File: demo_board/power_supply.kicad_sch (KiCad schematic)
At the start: 23 parts, among them J2 USB_C_Receptacle_USB2.0_16P, J3 BATT, U2 MCP73871-2CC, U3 AP2112K-3.3

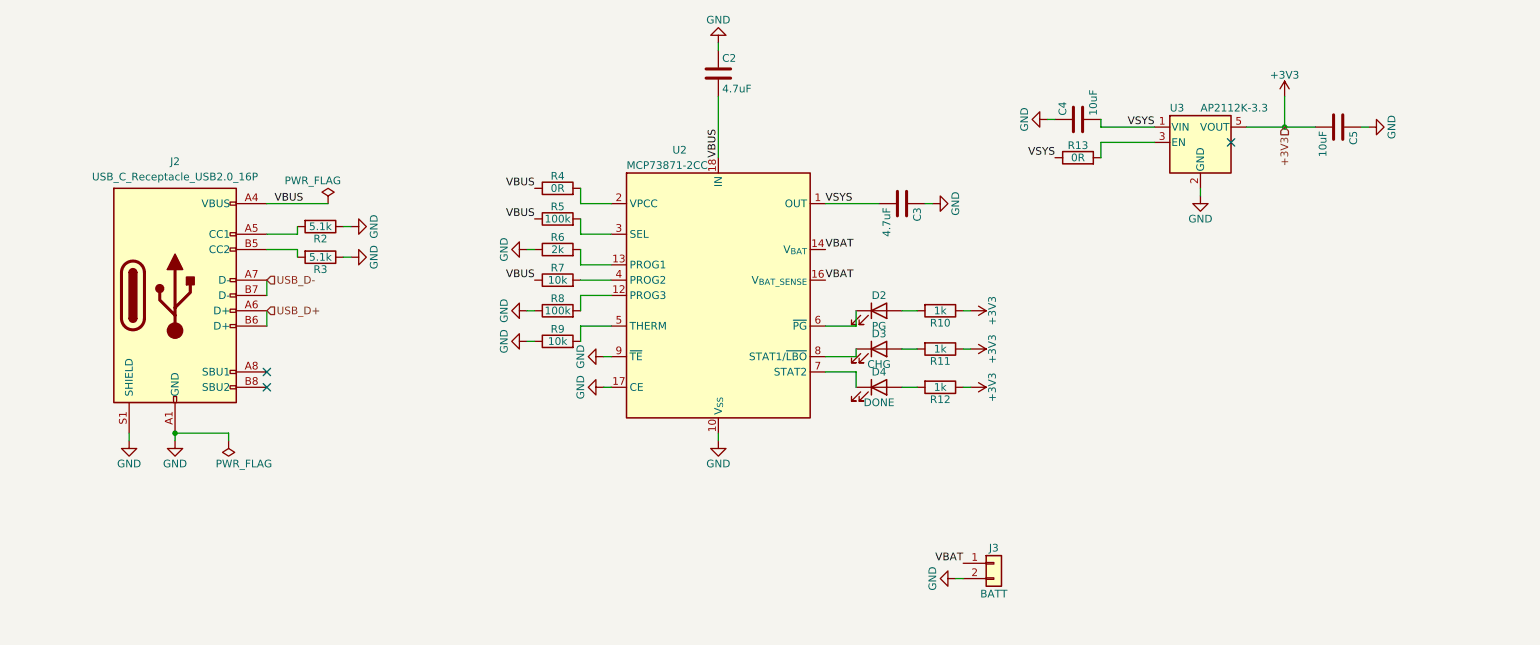
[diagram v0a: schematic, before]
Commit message: new demo board
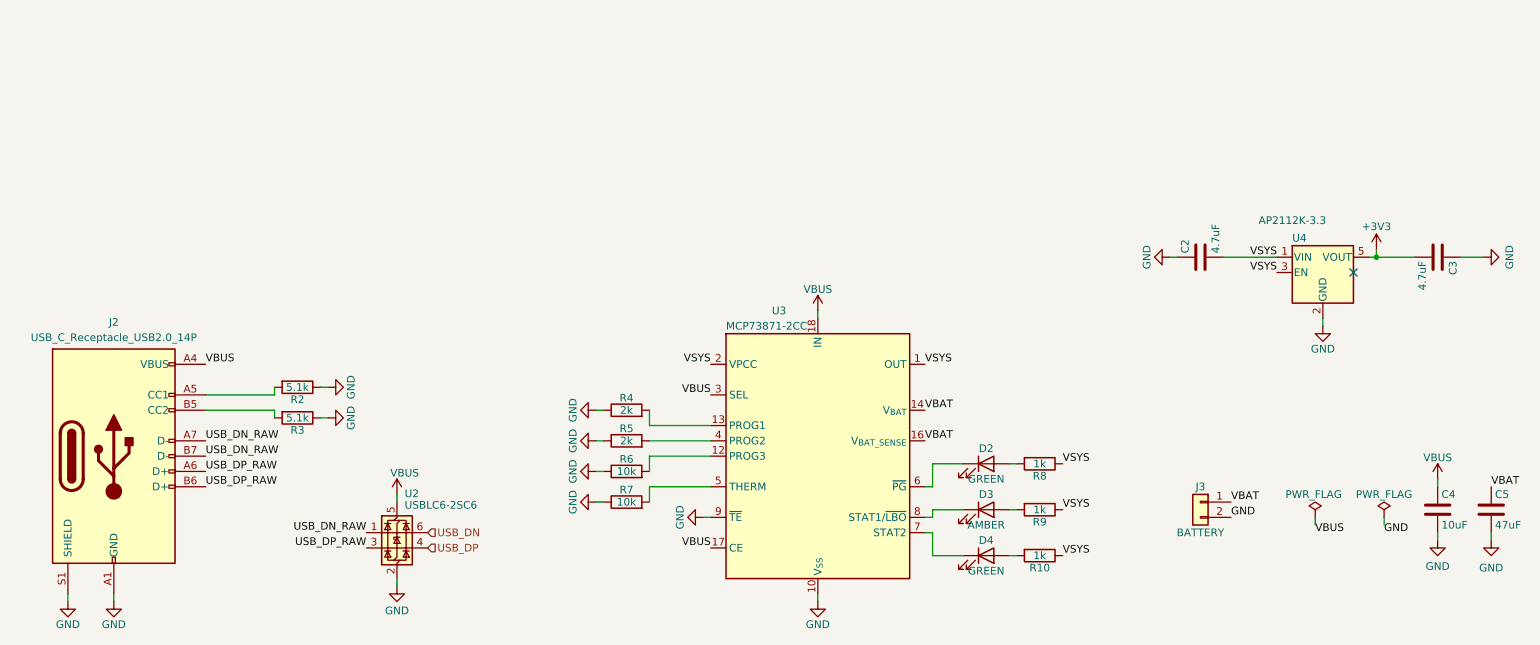
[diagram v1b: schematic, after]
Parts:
- removed J2: USB_C_Receptacle_USB2.0_16P, Connector_USB:USB_C_Receptacle_HRO_TYPE-C-31-M-12, symbol Connector:USB_C_Receptacle_USB2.0_16P
- removed R11, R12: 1k, Resistor_SMD:R_0402_1005Metric, symbol Device:R
- removed R13: 0R, Resistor_SMD:R_0402_1005Metric, symbol Device:R
- removed U2: MCP73871-2CC, Package_DFN_QFN:QFN-20-1EP_4x4mm_P0.5mm_EP2.5x2.5mm, symbol Battery_Management:MCP73871-2CC
- removed U3: AP2112K-3.3, Package_TO_SOT_SMD:SOT-23-5, symbol Regulator_Linear:AP2112K-3.3
- added J2: USB_C_Receptacle_USB2.0_14P, Connector_USB:USB_C_Receptacle_Amphenol_12401610E4-2A, symbol Connector:USB_C_Receptacle_USB2.0_14P
- added U2: USBLC6-2SC6, Package_TO_SOT_SMD:SOT-23-6, symbol Power_Protection:USBLC6-2SC6
- added U3: MCP73871-2CC, Package_DFN_QFN:QFN-20-1EP_4x4mm_P0.5mm_EP2.5x2.5mm, symbol Battery_Management:MCP73871
- added U4: AP2112K-3.3, Package_TO_SOT_SMD:SOT-23-5, symbol Regulator_Linear:AP2112K-3.3
- C2, C3: footprint Capacitor_SMD:C_0603_1608Metric -> Capacitor_SMD:C_0805_2012Metric
- C5: value 10uF -> 47uF; footprint Capacitor_SMD:C_0805_2012Metric -> Capacitor_SMD:C_1206_3216Metric
- D2: value PG -> GREEN
- D3: value CHG -> AMBER
- D4: value DONE -> GREEN
- J3: value BATT -> BATTERY
- R10, R2, R3, R7: footprint Resistor_SMD:R_0402_1005Metric -> Resistor_SMD:R_0603_1608Metric
- R4: value 0R -> 2k; footprint Resistor_SMD:R_0402_1005Metric -> Resistor_SMD:R_0603_1608Metric
- R5: value 100k -> 2k; footprint Resistor_SMD:R_0402_1005Metric -> Resistor_SMD:R_0603_1608Metric
- R6: value 2k -> 10k; footprint Resistor_SMD:R_0402_1005Metric -> Resistor_SMD:R_0603_1608Metric
- R8: value 100k -> 1k; footprint Resistor_SMD:R_0402_1005Metric -> Resistor_SMD:R_0603_1608Metric
- R9: value 10k -> 1k; footprint Resistor_SMD:R_0402_1005Metric -> Resistor_SMD:R_0603_1608Metric
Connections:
- net +3V3: now also C3.2, U4.5 (VOUT); no longer C5.2, R10.1
- net GND: now also C4.2, C5.2, R4.1, R5.1, R7.1, J2.A1 (GND), J2.A12 (GND), J2.B1 (GND), J2.B12 (GND), J2.S1 (SHIELD), U2.2 (GND), U3.10 (V_{SS}), U3.11 (V_{SS}), U3.21 (V_{SS}), U3.9 (~{TE}), U4.2 (GND); no longer C4.1, C5.1, R8.1, R9.1
- net VBAT: now also C5.1, U3.14 (V_{BAT}), U3.15 (V_{BAT}), U3.16 (V_{BAT_SENSE})
- net VBUS: now also C4.1, J2.A4 (VBUS), J2.A9 (VBUS), J2.B4 (VBUS), J2.B9 (VBUS), U2.5 (VBUS), U3.17 (CE), U3.18 (IN), U3.19 (IN), U3.3 (SEL); no longer C2.2, R4.1, R5.1, R7.1
- net VSYS: now also C2.2, R10.1, R8.1, R9.1, U3.1 (OUT), U3.2 (VPCC), U3.20 (OUT), U4.1 (VIN), U4.3 (EN); no longer C3.2, C4.2
- net at R5.2: now also U3.4 (PROG2)
- net at R7.2: now also U3.5 (THERM)
- net at R3.2: now also J2.B5 (CC2)
- net at R8.2: now also D2.2 (A)
- net at R2.2: now also J2.A5 (CC1)
- net at R4.2: now also U3.13 (PROG1)
- net at D3.1 (K): now also U3.8 (STAT1/~{LBO})
- net at D3.2 (A): now also R9.2
- net at D4.1 (K): now also U3.7 (STAT2)
- net at D4.2 (A): now also R10.2
- net at R6.2: now also U3.12 (PROG3)
- net at D2.1 (K): now also U3.6 (~{PG})
- new net USB_DN: U2.6 (I/O1)
- new net USB_DN_RAW: J2.A7 (D-), J2.B7 (D-), U2.1 (I/O1)
- new net USB_DP: U2.4 (I/O2)
- new net USB_DP_RAW: J2.A6 (D+), J2.B6 (D+), U2.3 (I/O2)
- no-connect marks 3 -> 1
